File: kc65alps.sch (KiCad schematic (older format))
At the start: 18 parts

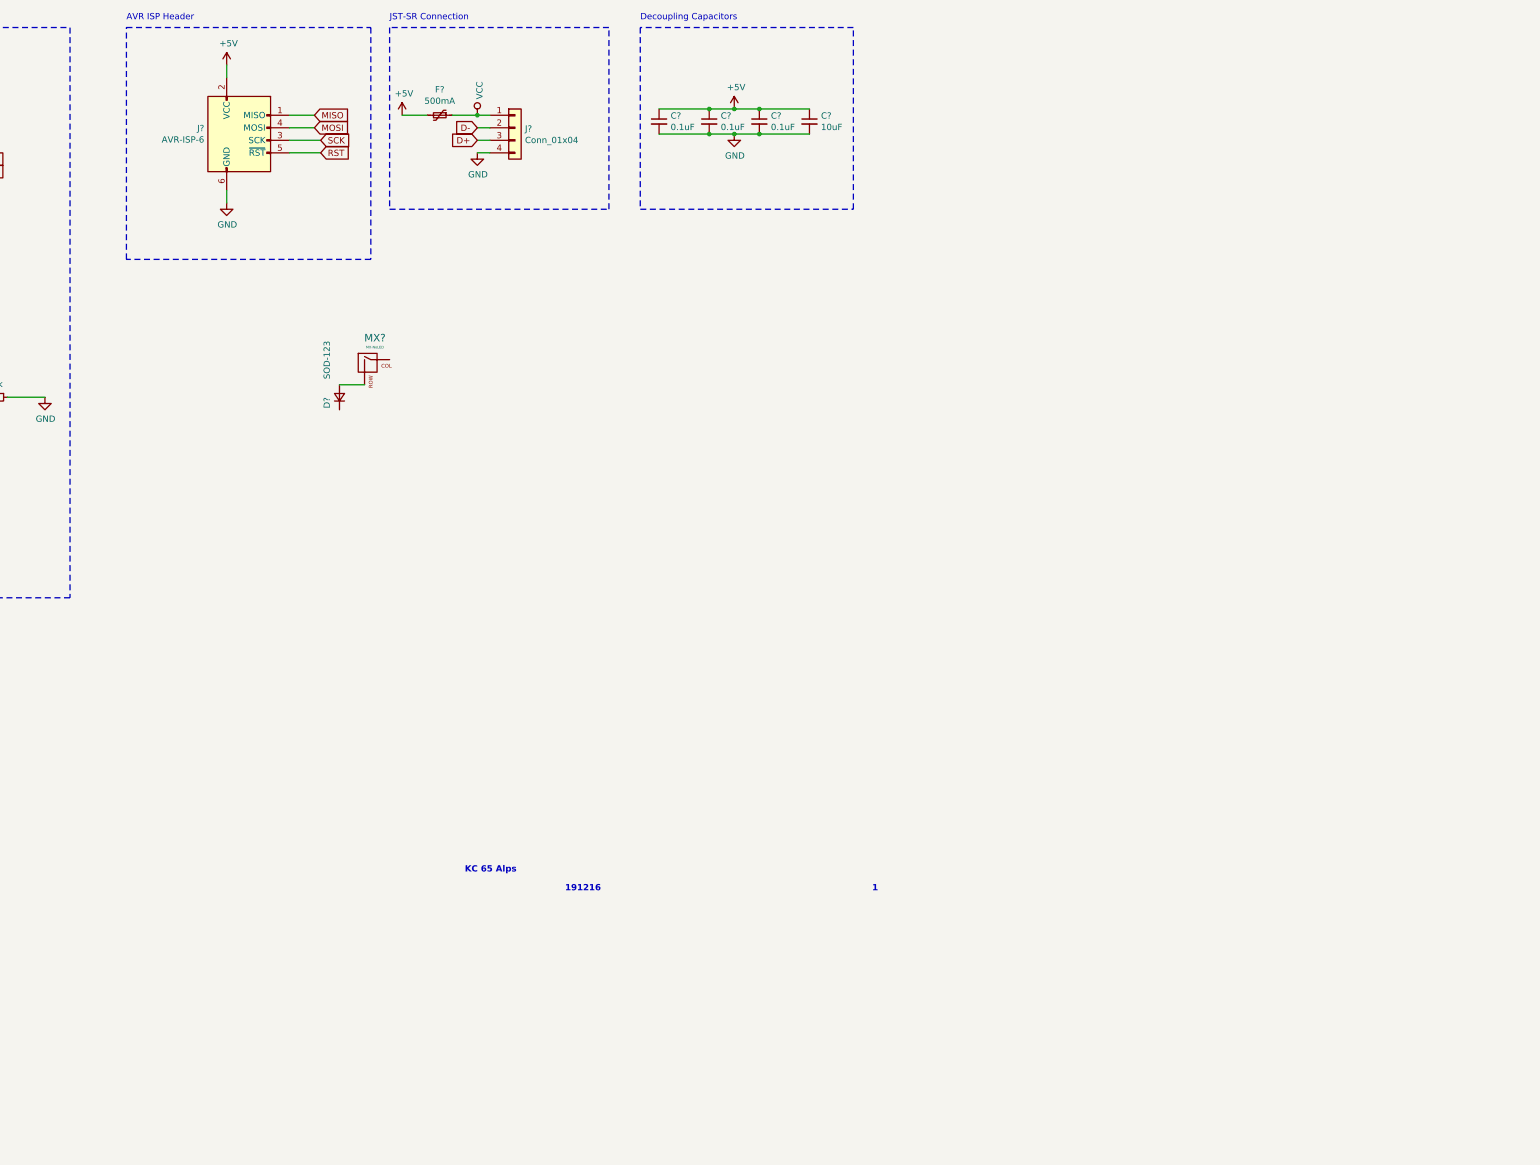
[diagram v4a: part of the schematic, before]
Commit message: Updating Schematic
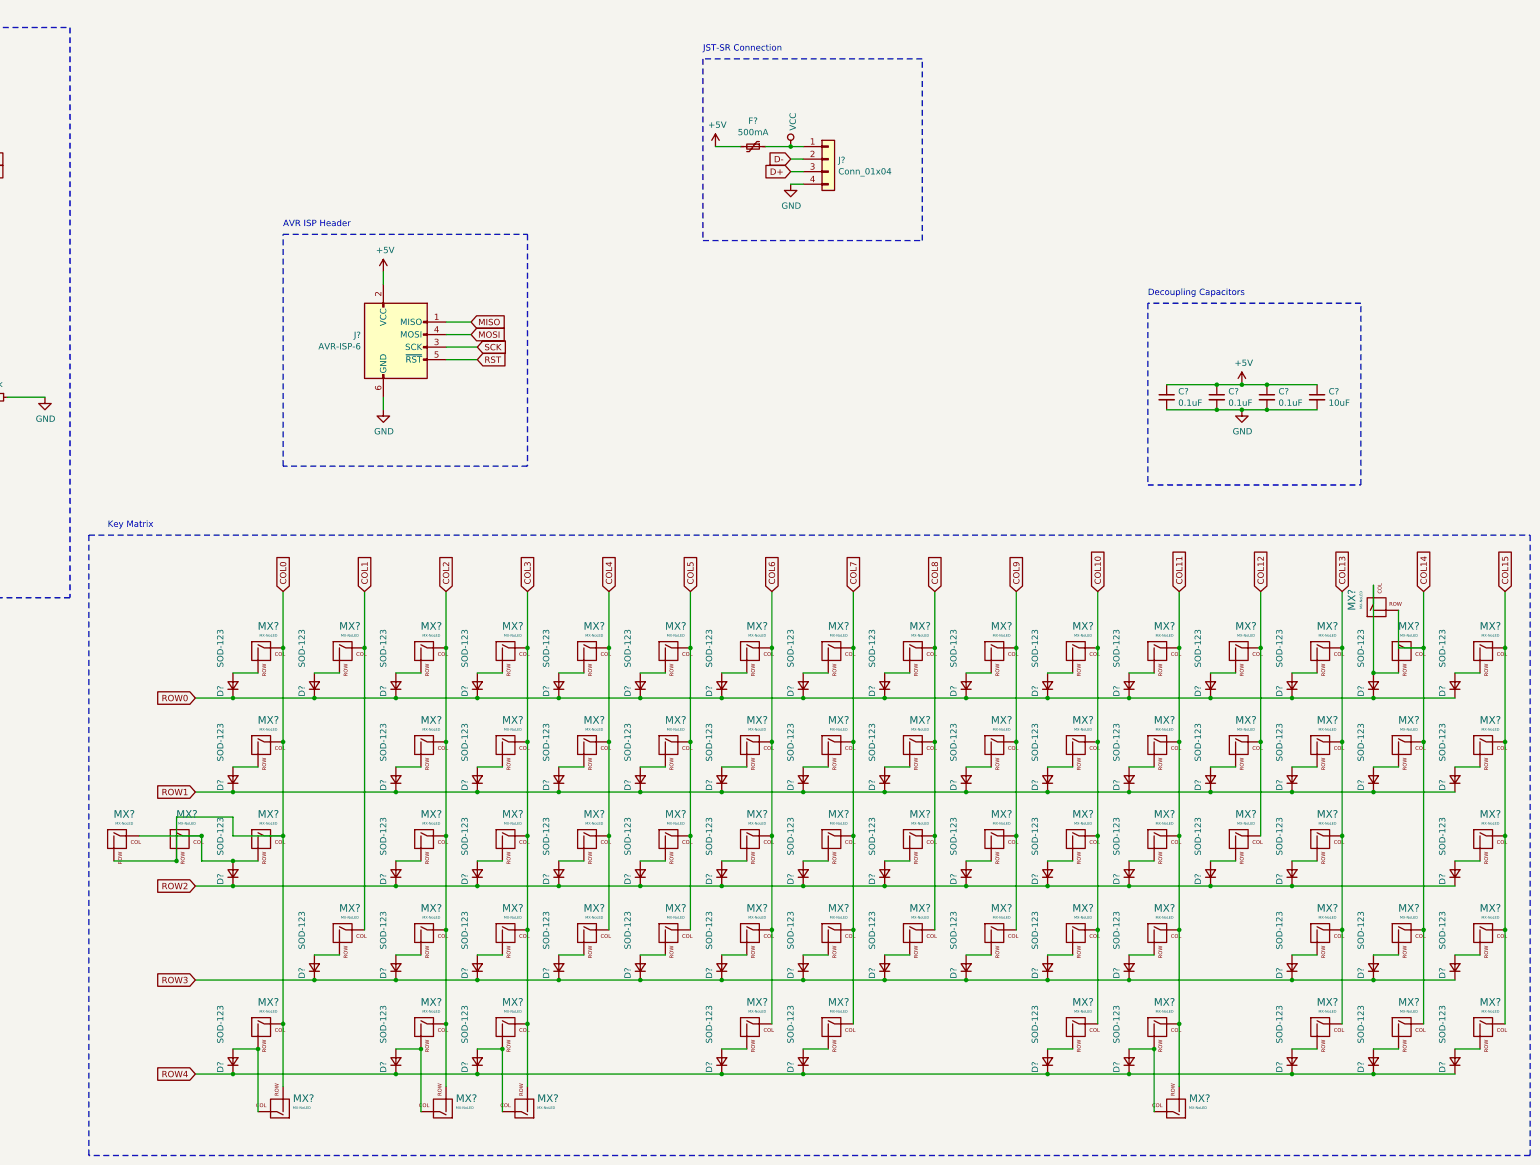
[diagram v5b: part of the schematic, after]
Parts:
- added D? (x68): SOD-123, symbol Device:D_Small
- added MX? (x75): MX-NoLED, symbol MX_Alps_Hybrid:MX-NoLED
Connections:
- net COL0: now reaches MX?.1 (COL)
- net COL0: now also MX?.1 (COL), MX?.1 (COL), MX?.1 (COL), MX?.2 (ROW), MX?.2 (ROW), MX?.2 (ROW)
- net ROW0: now reaches D?.1 (K)
- net ROW0: now also D?.1 (K), D?.1 (K), D?.1 (K), D?.1 (K), D?.1 (K), D?.1 (K), D?.1 (K), D?.1 (K), D?.1 (K), D?.1 (K), D?.1 (K), D?.1 (K), D?.1 (K), D?.1 (K), D?.1 (K)
- new net: D?.2 (A), MX?.2 (ROW) (x62)
- new net: D?.2 (A), MX?.1 (COL), MX?.2 (ROW) (x5)
- new net: D?.2 (A), MX?.1 (COL), MX?.1 (COL), MX?.2 (ROW)
- new net COL1: MX?.1 (COL), MX?.1 (COL)
- new net COL10: MX?.1 (COL), MX?.1 (COL), MX?.1 (COL), MX?.1 (COL), MX?.1 (COL)
- new net COL11: MX?.1 (COL), MX?.1 (COL), MX?.1 (COL), MX?.1 (COL), MX?.1 (COL), MX?.2 (ROW)
- new net COL12: MX?.1 (COL), MX?.1 (COL), MX?.1 (COL)
- new net COL13: MX?.1 (COL), MX?.1 (COL), MX?.1 (COL), MX?.1 (COL), MX?.1 (COL)
- new net COL14: MX?.1 (COL), MX?.1 (COL), MX?.1 (COL), MX?.1 (COL), MX?.2 (ROW)
- new net COL15: MX?.1 (COL), MX?.1 (COL), MX?.1 (COL), MX?.1 (COL), MX?.1 (COL)
- new net COL2: MX?.1 (COL), MX?.1 (COL), MX?.1 (COL), MX?.1 (COL), MX?.1 (COL), MX?.2 (ROW)
- new net COL3: MX?.1 (COL), MX?.1 (COL), MX?.1 (COL), MX?.1 (COL), MX?.1 (COL), MX?.2 (ROW)
- new net COL4: MX?.1 (COL), MX?.1 (COL), MX?.1 (COL), MX?.1 (COL)
- new net COL5: MX?.1 (COL), MX?.1 (COL), MX?.1 (COL), MX?.1 (COL)
- new net COL6: MX?.1 (COL), MX?.1 (COL), MX?.1 (COL), MX?.1 (COL), MX?.1 (COL)
- new net COL7: MX?.1 (COL), MX?.1 (COL), MX?.1 (COL), MX?.1 (COL), MX?.1 (COL)
- new net COL8: MX?.1 (COL), MX?.1 (COL), MX?.1 (COL), MX?.1 (COL)
- new net COL9: MX?.1 (COL), MX?.1 (COL), MX?.1 (COL), MX?.1 (COL)
- new net ROW1: D?.1 (K), D?.1 (K), D?.1 (K), D?.1 (K), D?.1 (K), D?.1 (K), D?.1 (K), D?.1 (K), D?.1 (K), D?.1 (K), D?.1 (K), D?.1 (K), D?.1 (K), D?.1 (K), D?.1 (K)
- new net ROW2: D?.1 (K), D?.1 (K), D?.1 (K), D?.1 (K), D?.1 (K), D?.1 (K), D?.1 (K), D?.1 (K), D?.1 (K), D?.1 (K), D?.1 (K), D?.1 (K), D?.1 (K), D?.1 (K)
- new net ROW3: D?.1 (K), D?.1 (K), D?.1 (K), D?.1 (K), D?.1 (K), D?.1 (K), D?.1 (K), D?.1 (K), D?.1 (K), D?.1 (K), D?.1 (K), D?.1 (K), D?.1 (K), D?.1 (K)
- new net ROW4: D?.1 (K), D?.1 (K), D?.1 (K), D?.1 (K), D?.1 (K), D?.1 (K), D?.1 (K), D?.1 (K), D?.1 (K), D?.1 (K)
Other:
- note added: "Key Matrix"
- note removed: "1"
- note removed: "191216"
- note removed: "KC 65 Alps"
- moved on the sheet: C?, D?, F?, J?, MX?
